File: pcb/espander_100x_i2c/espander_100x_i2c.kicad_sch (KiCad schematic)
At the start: 2 parts, among them U1 MCP23017_ML, U2 MCP23017_ML

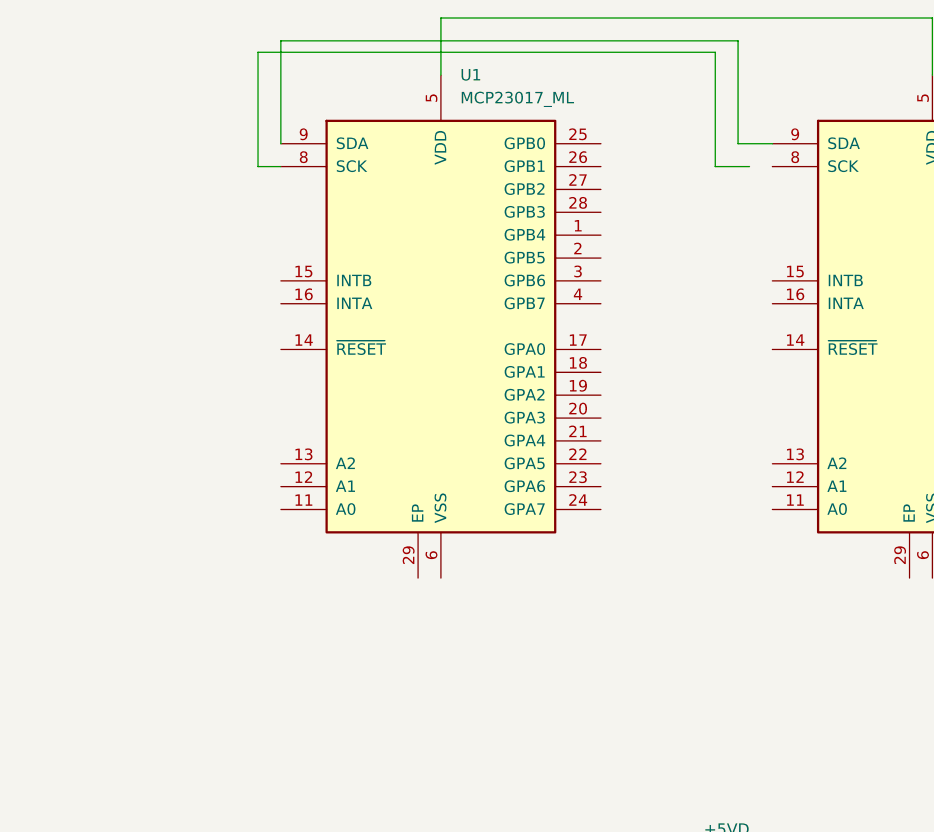
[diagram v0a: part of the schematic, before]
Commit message: Add backup of espander_100x_i2c project files from January 3, 2026
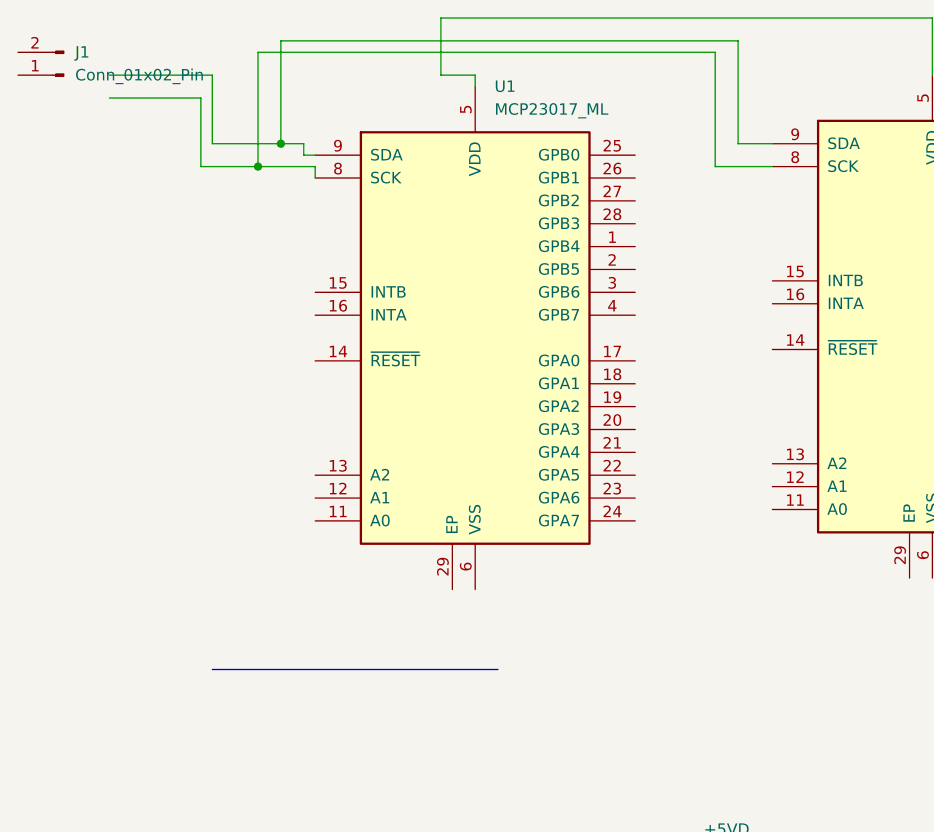
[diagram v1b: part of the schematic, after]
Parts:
- added J1: Conn_01x02_Pin, Connector_PinHeader_1.00mm:PinHeader_1x02_P1.00mm_Horizontal, symbol Connector:Conn_01x02_Pin
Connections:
- net at U2.8 (SCK): now also U1.8 (SCK)
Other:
- moved on the sheet: U1
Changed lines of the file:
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@@
 	(generator_version "9.0")
 	(paper "A4")
+	(junction
+		(at 35.56 33.02)
+		(diameter 0)
+		(color 0 0 0 0)
+	)
+	(junction
+		(at 38.1 30.48)
+		(diameter 0)
+		(color 0 0 0 0)
+	)
 	(wire
 		(pts
@@
 	(wire
 		(pts
+			(xy 41.91 33.02) (xy 41.91 34.29)
+		)
+		(stroke
+			(width 0)
+			(type default)
+		)
+	)
+	(wire
+		(pts
 			(xy 86.36 20.32) (xy 35.56 20.32)
 		)
@@
 	(wire
 		(pts
+			(xy 19.05 25.4) (xy 29.21 25.4)
+		)
+		(stroke
+			(width 0)
+			(type default)
+		)
+	)
+	(wire
+		(pts
+			(xy 30.48 30.48) (xy 38.1 30.48)
+		)
+		(stroke
+			(width 0)
+			(type default)
+		)
+	)
+	(wire
+		(pts
 			(xy 110.49 16.51) (xy 110.49 22.86)
 		)
@@
 	(wire
 		(pts
+			(xy 55.88 22.86) (xy 59.69 22.86)
+		)
+		(stroke
+			(width 0)
+			(type default)
+		)
+	)
+	(wire
+		(pts
 			(xy 55.88 16.51) (xy 110.49 16.51)
 		)
@@
 	(wire
 		(pts
+			(xy 19.05 22.86) (xy 30.48 22.86)
+		)
+		(stroke
+			(width 0)
+			(type default)
+		)
+	)
+	(wire
+		(pts
+			(xy 59.69 22.86) (xy 59.69 24.13)
+		)
+		(stroke
+			(width 0)
+			(type default)
+		)
+	)
+	(wire
+		(pts
+			(xy 29.21 25.4) (xy 29.21 33.02)
+		)
+		(stroke
+			(width 0)
+			(type default)
+		)
+	)
+	(wire
+		(pts
 			(xy 86.36 33.02) (xy 86.36 20.32)
 		)
@@
 	(wire
 		(pts
-			(xy 35.56 33.02) (xy 38.1 33.02)
+			(xy 35.56 33.02) (xy 41.91 33.02)
 		)
 		(stroke
@@
 	(wire
 		(pts
-			(xy 90.17 33.02) (xy 86.36 33.02)
+			(xy 86.36 33.02) (xy 92.71 33.02)
 		)
 		(stroke
@@
 		)
 	)
+	(bus
+		(pts
+			(xy 30.48 88.9) (xy 62.23 88.9)
+		)
+		(stroke
+			(width 0)
+			(type default)
+		)
+	)
+	(wire
+		(pts
+			(xy 29.21 33.02) (xy 35.56 33.02)
+		)
+		(stroke
+			(width 0)
+			(type default)
+		)
+	)
 	(wire
 		(pts
 			(xy 38.1 19.05) (xy 88.9 19.05)
+		)
+		(stroke
+			(width 0)
+			(type default)
+		)
+	)
+	(wire
+		(pts
+			(xy 30.48 22.86) (xy 30.48 30.48)
+		)
+		(stroke
+			(width 0)
+			(type default)
+		)
+	)
+	(wire
+		(pts
+			(xy 40.64 31.75) (xy 41.91 31.75)
+		)
+		(stroke
+			(width 0)
+			(type default)
+		)
+	)
+	(wire
+		(pts
+			(xy 40.64 30.48) (xy 40.64 31.75)
+		)
+		(stroke
+			(width 0)
+			(type default)
+		)
+	)
+	(wire
+		(pts
+			(xy 38.1 30.48) (xy 40.64 30.48)
 		)
 		(stroke
@@
 	)
 	(symbol
+		(lib_id "Connector:Conn_01x02_Pin")
+		(at 13.97 22.86 180)
+		(unit 1)
+		(exclude_from_sim no)
+		(in_bom yes)
+		(on_board yes)
+		(dnp no)
+		(fields_autoplaced yes)
+		(property "Reference" "J1"
+			(at 15.24 20.3199 0)
+			(effects
+				(font
+					(size 1.27 1.27)
+				)
+				(justify right)
+			)
+		)
+		(property "Value" "Conn_01x02_Pin"
+			(at 15.24 22.8599 0)
+			(effects
+				(font
+					(size 1.27 1.27)
+				)
+				(justify right)
+			)
+		)
+		(property "Footprint" "Connector_PinHeader_1.00mm:PinHeader_1x02_P1.00mm_Horizontal"
+			(at 13.97 22.86 0)
+			(effects
+				(font
+					(size 1.27 1.27)
+				)
+				(hide yes)
+			)
+		)
+		(property "Datasheet" "~"
+			(at 13.97 22.86 0)
+			(effects
+				(font
+					(size 1.27 1.27)
+				)
+				(hide yes)
+			)
+		)
+		(property "Description" "Generic connector, single row, 01x02, script generated"
+			(at 13.97 22.86 0)
+			(effects
+				(font
+					(size 1.27 1.27)
+				)
+				(hide yes)
+			)
+		)
+		(pin "2"
+		)
+		(pin "1"
+		)
+		(instances
+			(project ""
+				(path "/824ceec5-564f-405b-8bea-e5a9f7aa2926"
+					(reference "J1")
+					(unit 1)
+				)
+			)
+		)
+	)
+	(symbol
 		(lib_id "power:GND")
 		(at 93.98 111.76 0)
@@
 	(symbol
 		(lib_id "Interface_Expansion:MCP23017_ML")
-		(at 55.88 50.8 0)
+		(at 59.69 52.07 0)
 		(unit 1)
 		(exclude_from_sim no)
@@
 		(fields_autoplaced yes)
 		(property "Reference" "U1"
-			(at 58.0233 22.86 0)
+			(at 61.8333 24.13 0)
 			(effects
 				(font
@@
 		)
 		(property "Value" "MCP23017_ML"
-			(at 58.0233 25.4 0)
+			(at 61.8333 26.67 0)
 			(effects
 				(font
@@
 		)
 		(property "Footprint" "Package_DFN_QFN:QFN-28-1EP_6x6mm_P0.65mm_EP4.25x4.25mm"
-			(at 60.96 76.2 0)
+			(at 64.77 77.47 0)
 			(effects
 				(font
@@
 		)
 		(property "Datasheet" "https://ww1.microchip.com/downloads/aemDocuments/documents/APID/ProductDocuments/DataSheets/MCP23017-Data-Sheet-DS20001952.pdf"
-			(at 60.96 78.74 0)
+			(at 64.77 80.01 0)
 			(effects
 				(font
@@
 		)
 		(property "Description" "16-bit I/O expander, I2C, interrupts, w pull-ups, GPA/B7 output only (https://microchip.my.site.com/s/article/GPA7---GPB7-Cannot-Be-Used-as-Inputs-In-MCP23017), QFN-28"
-			(at 55.88 50.8 0)
-			(effects
-				(font
+			(at 59.69 52.07 0)
+			(effects
+				(font

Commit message: Refactor code structure and remove redundant sections for improved readability and maintainability
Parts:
- removed J1: Conn_01x02_Pin, Connector_PinHeader_1.00mm:PinHeader_1x02_P1.00mm_Horizontal, symbol Connector:Conn_01x02_Pin
- removed U1, U2: MCP23017_ML, Package_DFN_QFN:QFN-28-1EP_6x6mm_P0.65mm_EP4.25x4.25mm, symbol Interface_Expansion:MCP23017_ML
- added J1, J10, J11, J12, J13, J14, J15, J16, J17, J18, J19, J2, J20, J3, J4, J5, J6, J7, J8, J9: DG127A-5.08-06P-14-00AH, DG127A50806P1400AH, symbol 1_tme:DG127A-5.08-06P-14-00AH
- added U1, U2, U3, U4, U5, U6, U7: MCP23017_SP, Package_DIP:DIP-28_W7.62mm, symbol Interface_Expansion:MCP23017_SP
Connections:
- new net: U1.10 (VSS), U2.10 (VSS), U3.10 (VSS), U4.10 (VSS), U5.10 (VSS), U6.10 (VSS), U7.10 (VSS)
- new net: U1.12 (SCK), U2.12 (SCK), U3.12 (SCK), U4.12 (SCK), U5.12 (SCK), U6.12 (SCK), U7.12 (SCK)
- new net: U1.13 (SDA), U2.13 (SDA), U3.13 (SDA), U4.13 (SDA), U5.13 (SDA), U6.13 (SDA), U7.13 (SDA)
- new net: U1.9 (VDD), U2.9 (VDD), U3.9 (VDD), U4.9 (VDD), U5.9 (VDD), U6.9 (VDD), U7.9 (VDD)
- new net: J11.1, U1.7 (GPB6)
- new net: J11.2, U1.8 (GPB7)
- new net: J11.3, U1.21 (GPA0)
- new net: J11.4, U1.22 (GPA1)
- new net: J11.5, U1.23 (GPA2)
- new net: J11.6, U1.24 (GPA3)
- new net: J1.1, U1.1 (GPB0)
- new net: J1.2, U1.2 (GPB1)
- new net: J1.3, U1.3 (GPB2)
- new net: J1.4, U1.4 (GPB3)
- new net: J1.5, U1.5 (GPB4)
- new net: J1.6, U1.6 (GPB5)
